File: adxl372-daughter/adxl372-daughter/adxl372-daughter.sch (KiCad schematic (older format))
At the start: 8 parts, among them J1 Conn_01x08, J2 Conn_01x08, J3 Conn_01x05_Female, J4 Conn_01x05_Female, U1 ADXL372

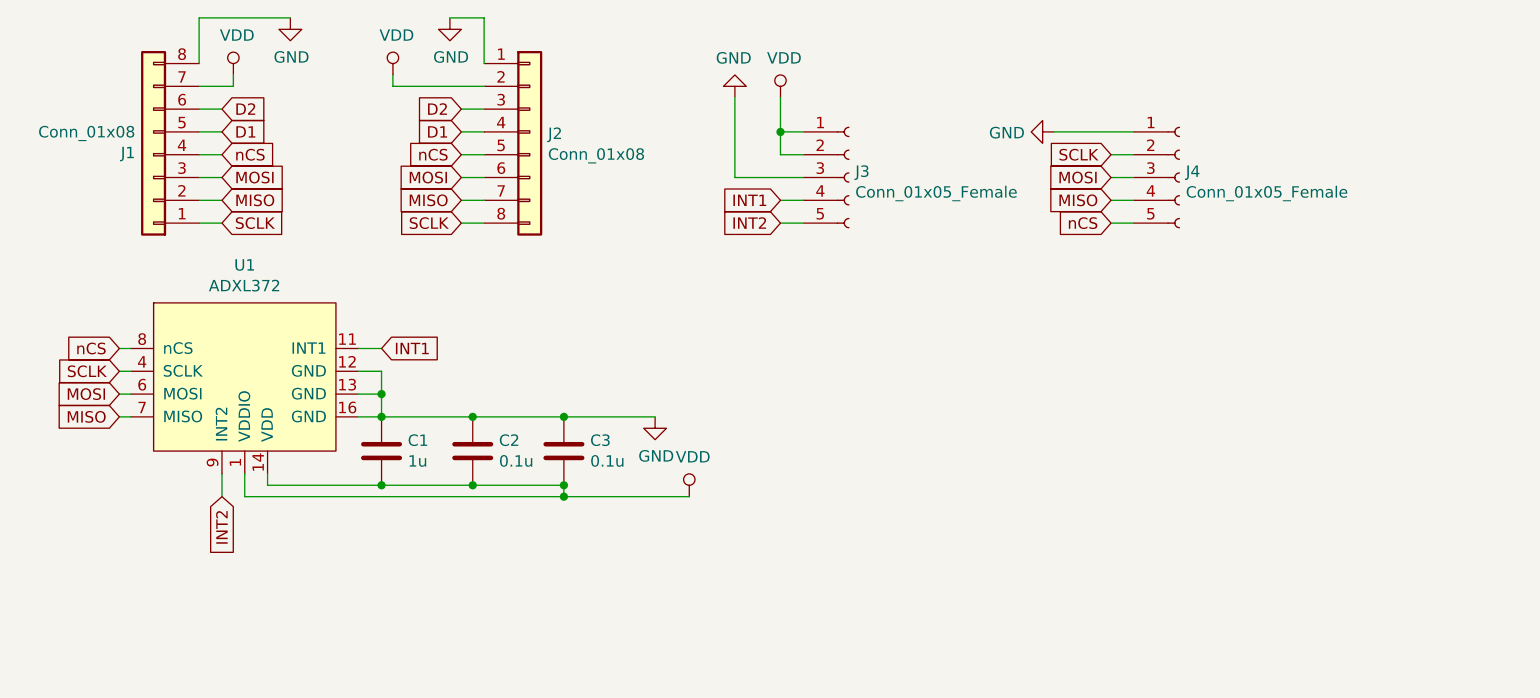
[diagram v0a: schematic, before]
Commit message: fleshed out daughter card
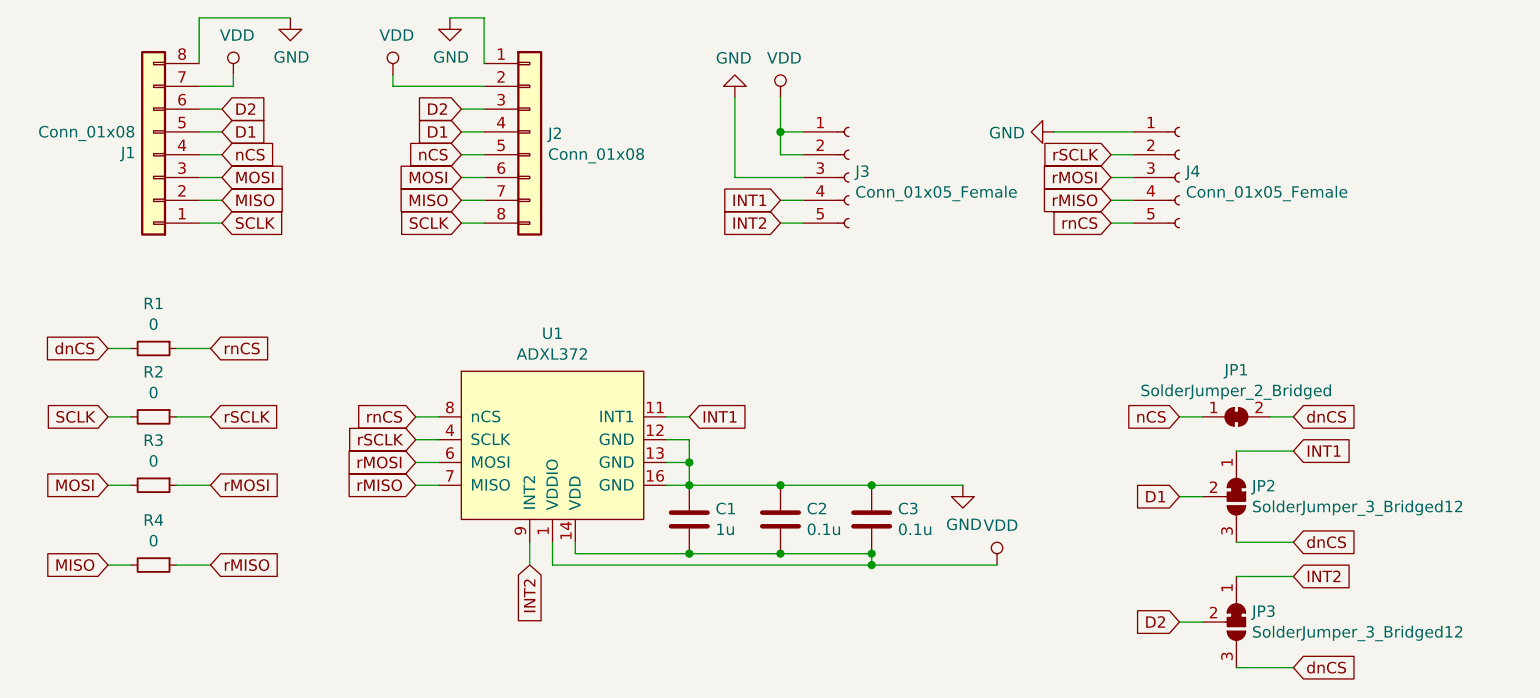
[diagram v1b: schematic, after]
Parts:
- added JP1: SolderJumper_2_Bridged, Jumper:SolderJumper-2_P1.3mm_Bridged2Bar_Pad1.0x1.5mm, symbol Jumper:SolderJumper_2_Bridged
- added JP2, JP3: SolderJumper_3_Bridged12, Jumper:SolderJumper-3_P1.3mm_Bridged2Bar12_Pad1.0x1.5mm, symbol Jumper:SolderJumper_3_Bridged12
- added R1, R2, R3, R4: 0, Resistor_SMD:R_0603_1608Metric_Pad1.05x0.95mm_HandSolder, symbol Device:R_Small
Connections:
- net D1: now also JP2.2 (C)
- net D2: now also JP3.2 (C)
- net INT1: now also JP2.1 (A)
- net INT2: now also JP3.1 (A)
- net MISO: now also R4.2; no longer J4.4 (Pin_4), U1.7 (MISO)
- net MOSI: now also R3.2; no longer J4.3 (Pin_3), U1.6 (MOSI)
- net SCLK: now also R2.2; no longer J4.2 (Pin_2), U1.4 (SCLK)
- net nCS: now also JP1.1 (A); no longer J4.5 (Pin_5), U1.8 (nCS)
- new net dnCS: JP1.2 (B), JP2.3 (B), JP3.3 (B), R1.2
- new net rMISO: J4.4 (Pin_4), R4.1, U1.7 (MISO)
- new net rMOSI: J4.3 (Pin_3), R3.1, U1.6 (MOSI)
- new net rSCLK: J4.2 (Pin_2), R2.1, U1.4 (SCLK)
- new net rnCS: J4.5 (Pin_5), R1.1, U1.8 (nCS)
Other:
- moved on the sheet: C1, C2, C3, U1
